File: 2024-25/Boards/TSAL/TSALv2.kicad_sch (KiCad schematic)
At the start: 26 parts, among them J1 043045-0412, Q1 BS250P, Q2 BS170, Q3 UJ3N120035K3S, Q4 BS170, U1 H11L1M, U2 NE555D

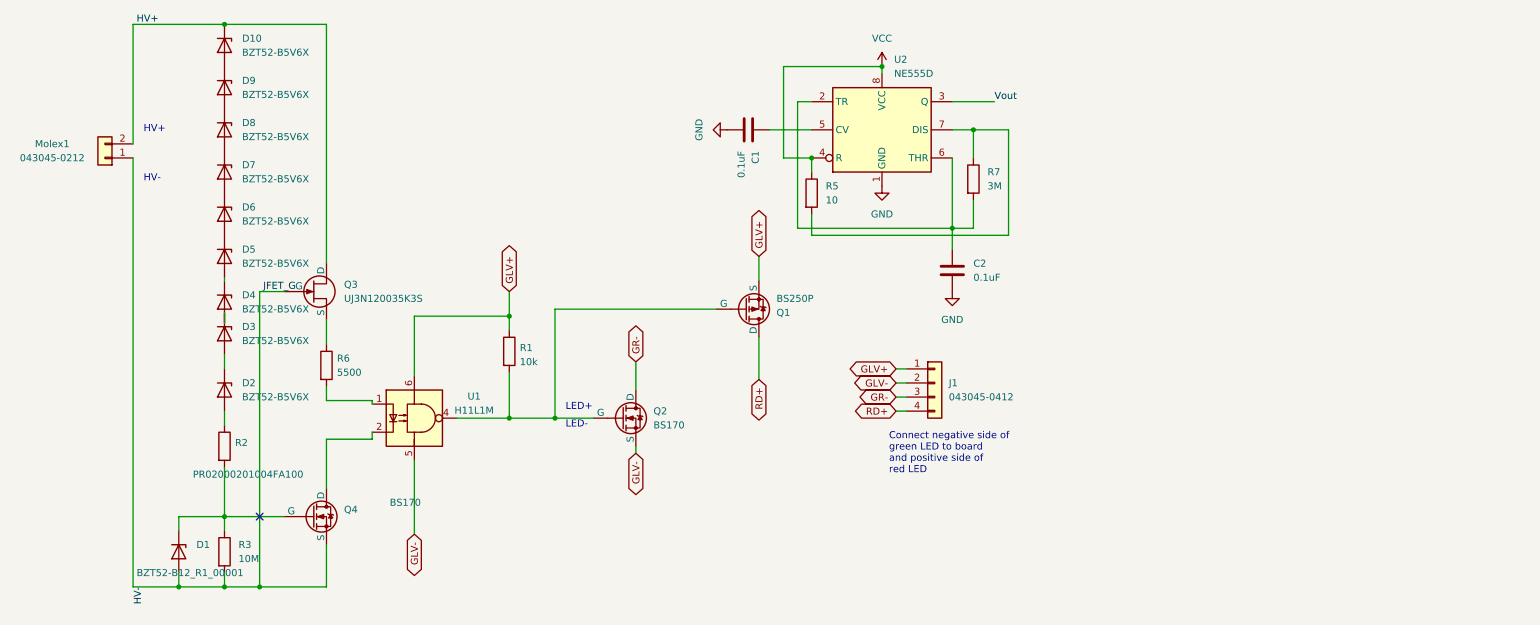
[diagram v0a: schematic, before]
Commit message: Board should be ready for pcb
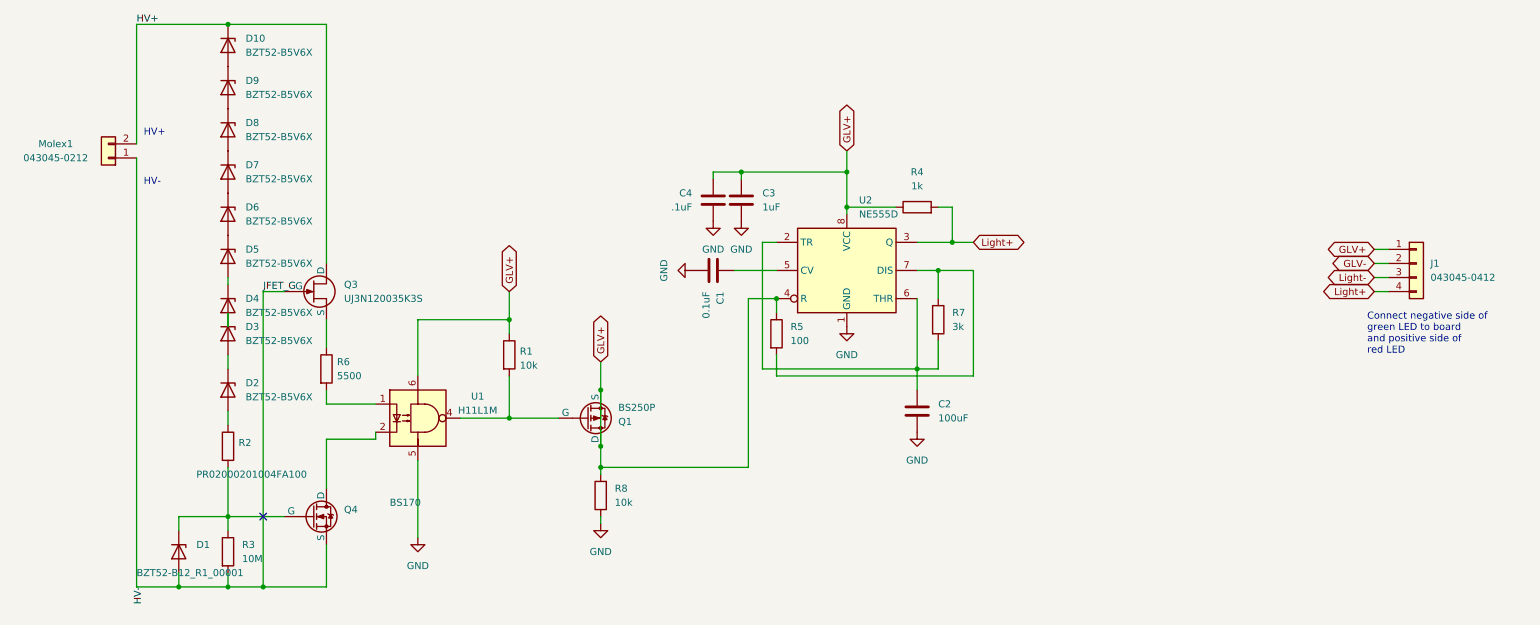
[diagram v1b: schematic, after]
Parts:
- removed Q2: BS170, Package_TO_SOT_THT:TO-92, symbol Simulation_SPICE:NMOS
- added C3: 1uF, Capacitor_SMD:C_0805_2012Metric_Pad1.18x1.45mm_HandSolder, symbol Device:C
- added C4: .1uF, Capacitor_SMD:C_0402_1005Metric_Pad0.74x0.62mm_HandSolder, symbol Device:C
- added R4: 1k, symbol Device:R
- added R8: 10k, symbol Device:R
- C2: value 0.1uF -> 100uF
- R5: value 10 -> 100
- R7: value 3M -> 3k
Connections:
- net VCC is gone; now on net GLV+: R5.1, U2.4 (R), U2.8 (VCC)
- net Vout is gone; now on net Light+: U2.3 (Q)
- net GLV+: now also Q1.1 (D), C3.2, C4.2, R4.1, R8.2
- net GLV-: no longer U1.5
- net GND: now also U1.5, C3.1, C4.1, R8.1
- net GR- renamed Light-
- net RD+ renamed Light+
- net Light+: now also R4.2; no longer Q1.1 (D)
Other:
- note removed: "LED+"
- note removed: "LED-"
- moved on the sheet: C1, C2, D10, D2, D3, D4, D5, D6, D7, D8, D9, J1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
